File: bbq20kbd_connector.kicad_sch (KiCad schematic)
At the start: 24 parts, among them J8 BBQ20KBD, Q1 BSS138, Q2 BSS138, Q3 BSS138, Q4 BSS138, Q5 BSS138, Q6 BSS138, U2 TPS7A2018PDBVR, U3 TPS7A2028PDBVR

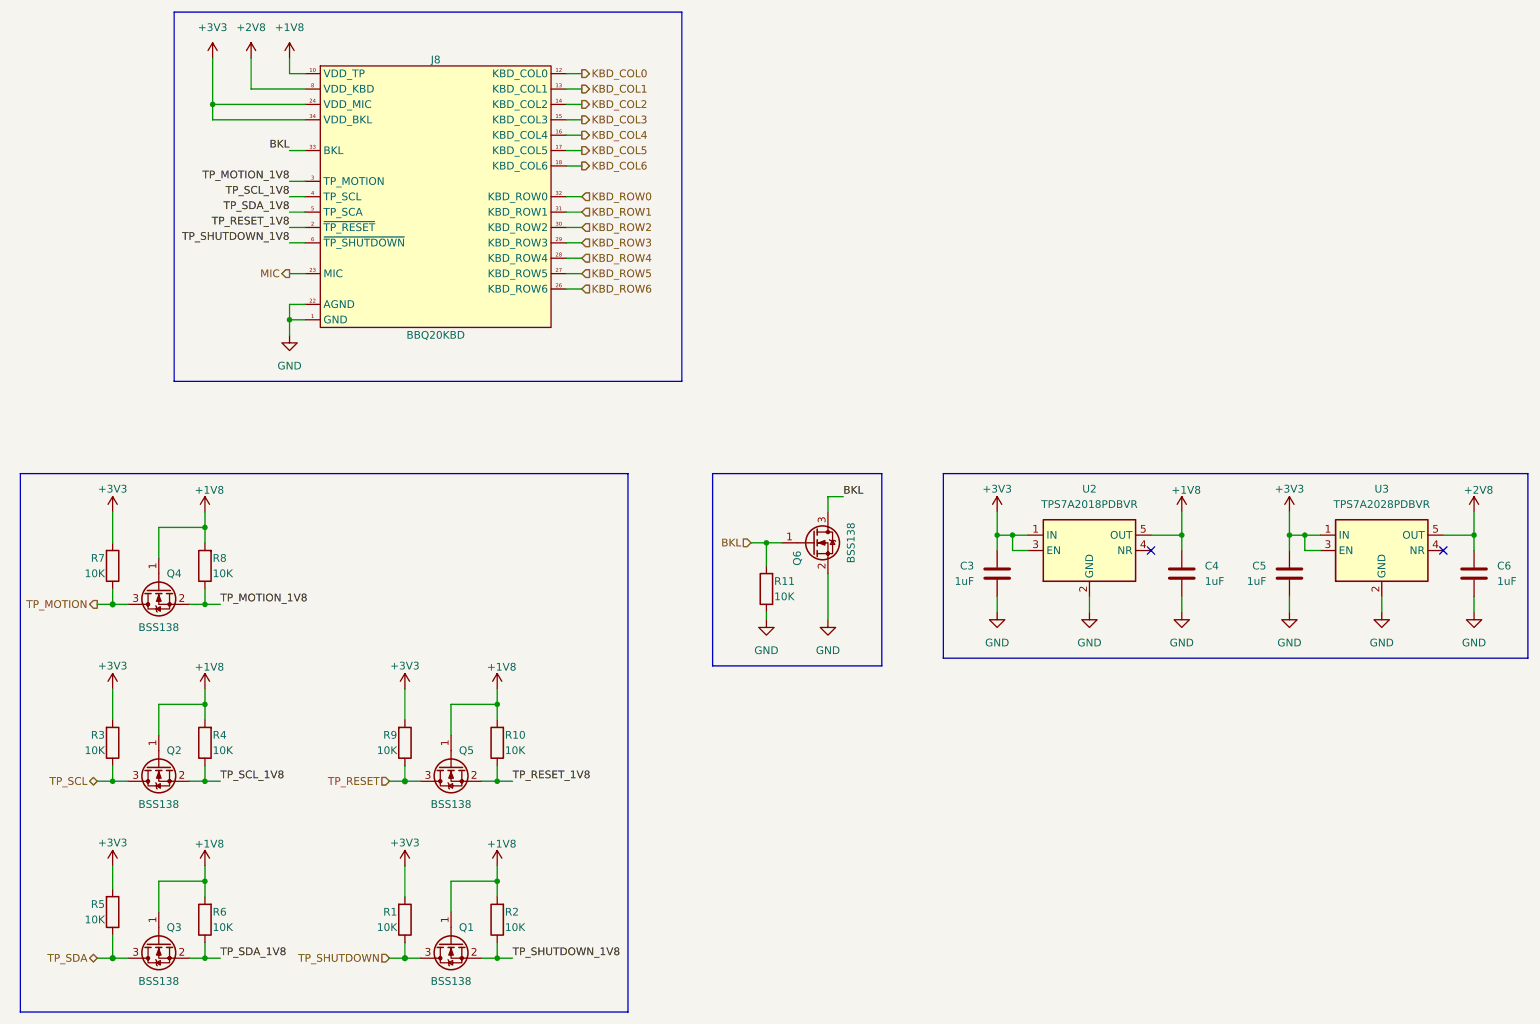
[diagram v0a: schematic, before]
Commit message: Version 1
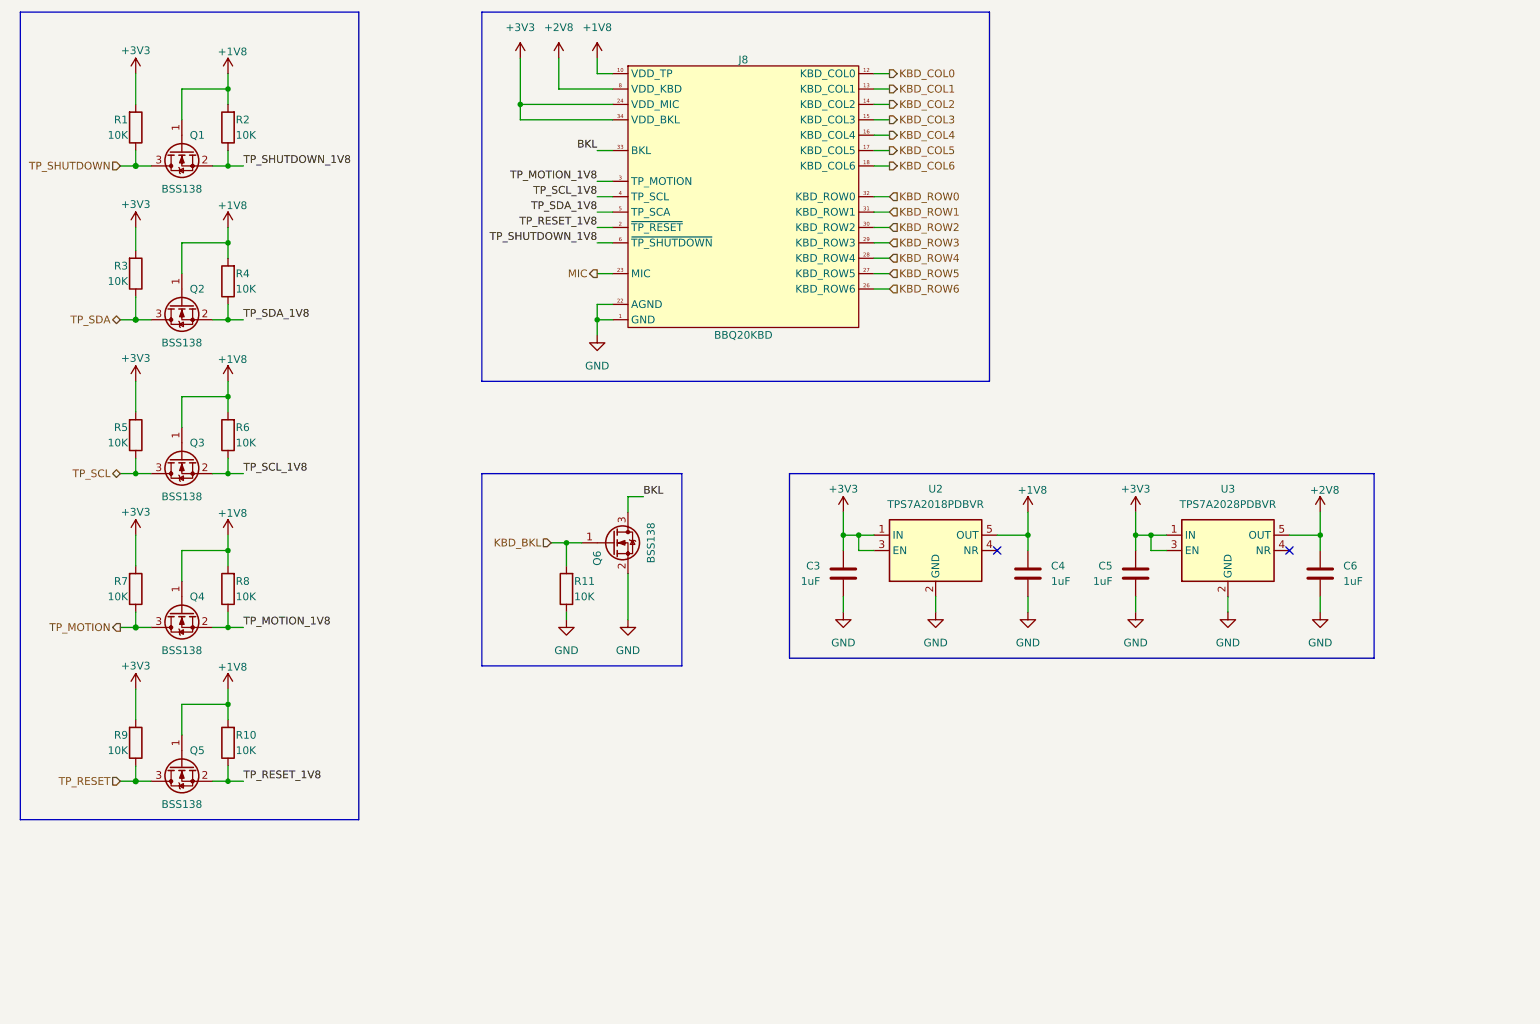
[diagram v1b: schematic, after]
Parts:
- renumbered Q3 to Q2, Q2 to Q3, R5 to R3, R6 to R4, R3 to R5, R4 to R6
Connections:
- net BKL: no longer Q6.1 (G), R11.2
- new net KBD_BKL: Q6.1 (G), R11.2
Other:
- moved on the sheet: C3, C4, C5, C6, J8, Q1, Q2, Q3, Q4, Q5, Q6, R1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
